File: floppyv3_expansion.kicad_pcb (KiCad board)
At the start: 2 copper layers, 69 x 84 mm, 15 parts, among them J101 Left_Bank_Board_Socket, J102 Right_Bank_Board_Socket, J103 FTSH-107-01-L-DV-K-TR, J104 STLink_Board_Conn, J105 Left_Bank_Free_Socket, J106 Right_Bank_Free_Socket, J107 POT_OUT, U101 MAX6816

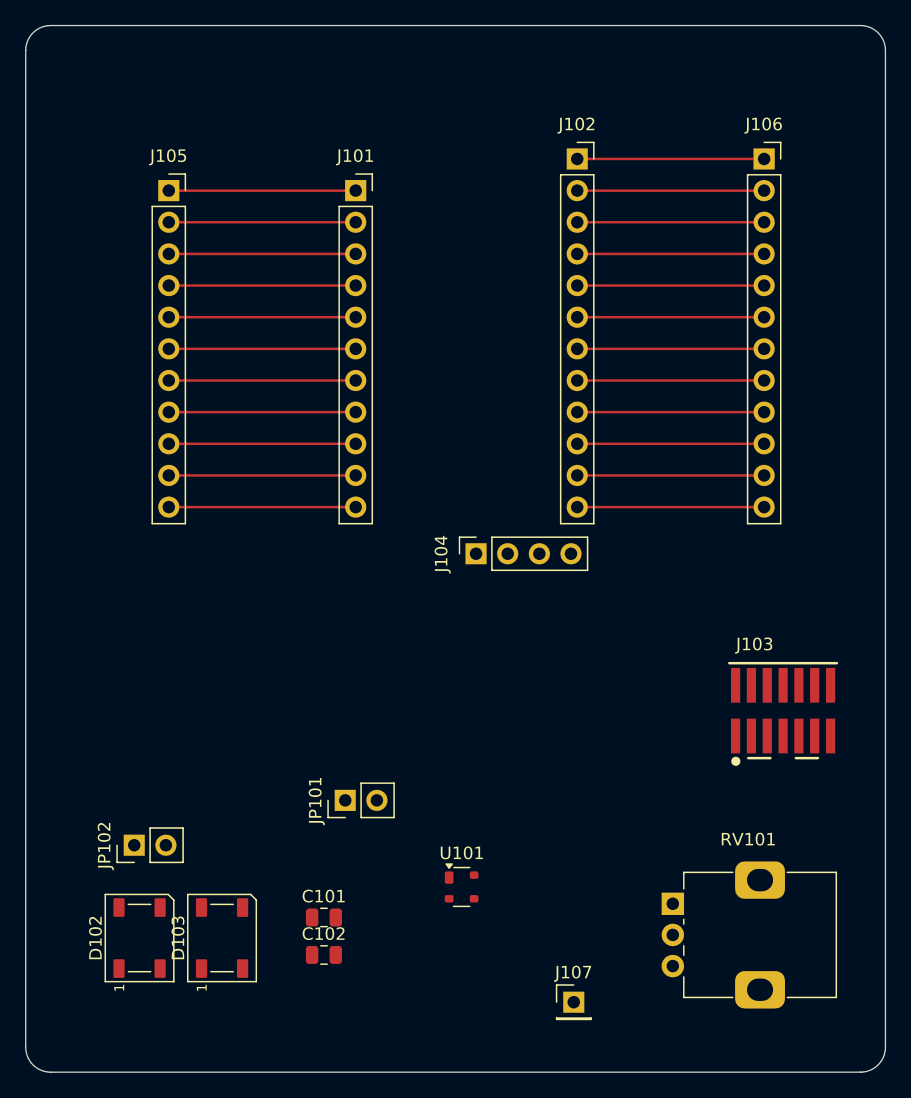
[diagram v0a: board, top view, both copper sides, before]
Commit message: Further improvements to layout and schematic
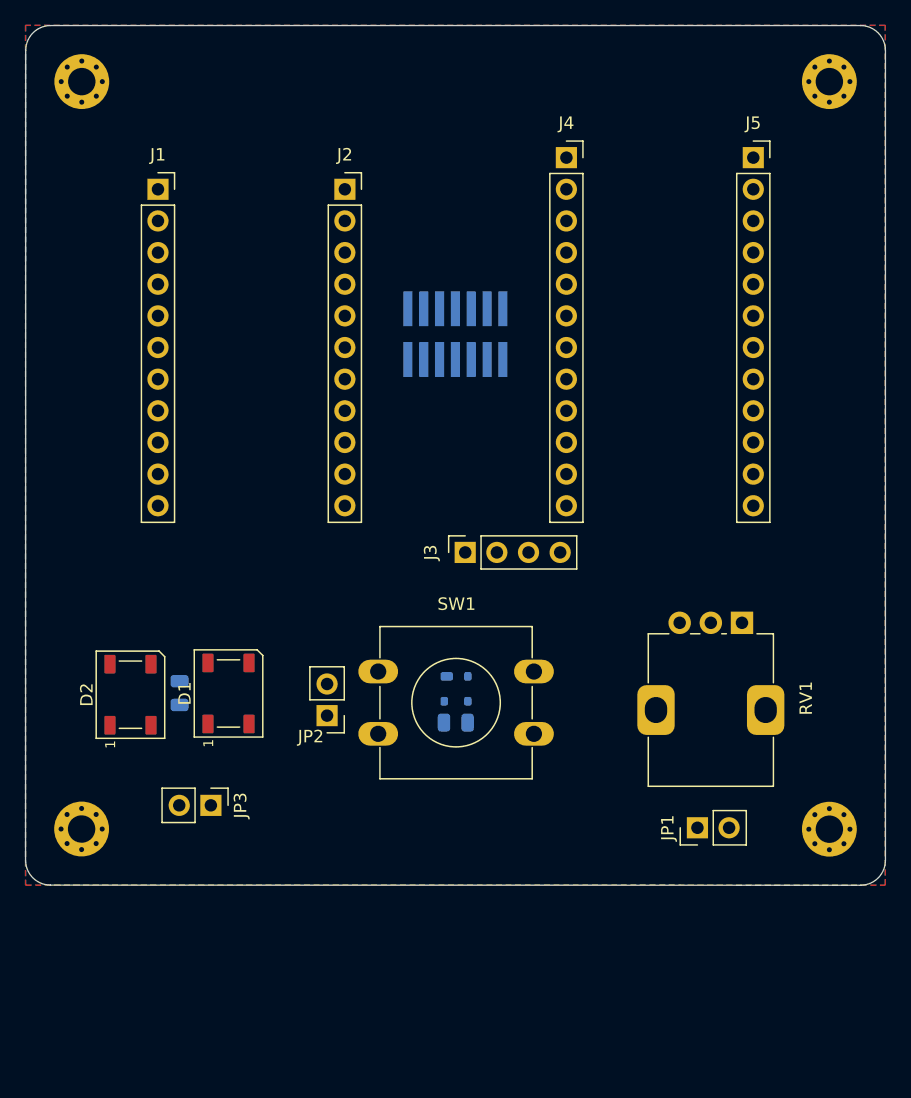
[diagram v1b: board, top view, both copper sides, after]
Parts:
- removed J107: POT_OUT, Connector_PinHeader_2.54mm:PinHeader_1x01_P2.54mm_Vertical
- added H1: MountingHole, MountingHole:MountingHole_2.2mm_M2_Pad_Via, F.Cu at (85.1, 68.9)
- added H2: MountingHole, MountingHole:MountingHole_2.2mm_M2_Pad_Via, F.Cu at (145.1, 68.9)
- added H3: MountingHole, MountingHole:MountingHole_2.2mm_M2_Pad_Via, F.Cu at (145.1, 128.9)
- added H4: MountingHole, MountingHole:MountingHole_2.2mm_M2_Pad_Via, F.Cu at (85.1, 128.9)
- added JP1: POT_JMP, Connector_PinHeader_2.54mm:PinHeader_1x02_P2.54mm_Vertical, F.Cu at (134.5, 128.8)
- added SW1: USR_BTN, Button_Switch_THT:SW_PUSH-12mm, F.Cu at (108.9, 116.3)
- C1: renamed from C101; moved to B.Cu
- C2: renamed from C102; moved to B.Cu
- J6: renamed from J103; moved to B.Cu
- U1: renamed from U101; moved to B.Cu
- moved J6 40.1 mm to (115.1, 89.2), turned to 180 degrees
- moved C2 24.0 mm to (93.0, 118.0), turned to -90 degrees
- moved RV1 23.2 mm to (138.1, 112.3), turned to -90 degrees
- moved D1 20.9 mm to (96.9, 118.0)
- moved D2 20.9 mm to (89.0, 118.1)
- moved C1 18.9 mm to (115.1, 120.4)
- moved U1 15.9 mm to (115.2, 117.7), turned to -90 degrees
- moved JP2 6.95 mm to (104.8, 119.8), turned to 180 degrees
- moved JP3 6.93 mm to (95.5, 127.0), turned to -90 degrees
- moved J5 0.88 mm to (139.0, 75.0)
- moved J3 0.88 mm to (115.9, 106.7)
- moved J1 0.88 mm to (91.2, 77.6)
- moved J2 0.88 mm to (106.2, 77.6)
- moved J4 0.88 mm to (124.0, 75.0)
- renumbered D102 to D1, D103 to D2, J105 to J1, J101 to J2, J104 to J3, J102 to J4, J106 to J5, JP101 to JP2, JP102 to JP3, RV101 to RV1
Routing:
- net GND: track 29.3 -> 0.00 mm
- net /VUSB: track 15.0 -> 0.00 mm
- net /VIN: track 15.0 -> 0.00 mm
- net /PB3: track 15.0 -> 0.00 mm
- net /PB0: track 15.0 -> 0.00 mm
- net /PA7: track 15.0 -> 0.00 mm
- net /PA6: track 15.0 -> 0.00 mm
- net /PA5: track 15.0 -> 0.00 mm
- net /PA14: track 15.0 -> 0.00 mm
- net /PA13: track 15.0 -> 0.00 mm
- net /PA12: track 15.0 -> 0.00 mm
- net /PA11: track 15.0 -> 0.00 mm
- net /PC15: track 14.3 -> 0.00 mm
- net /PC14: track 14.3 -> 0.00 mm
- net /PB7: track 14.3 -> 0.00 mm
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- added copper zone on B.Cu, net GND
- added copper zone on F.Cu, net GND
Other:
- board size 69 x 84 mm -> 69 x 69 mm
